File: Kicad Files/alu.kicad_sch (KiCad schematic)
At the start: 27 parts, among them U47 74LS245, U48 74LS283, U49 74LS283, U50 74LS86, U51 74LS86

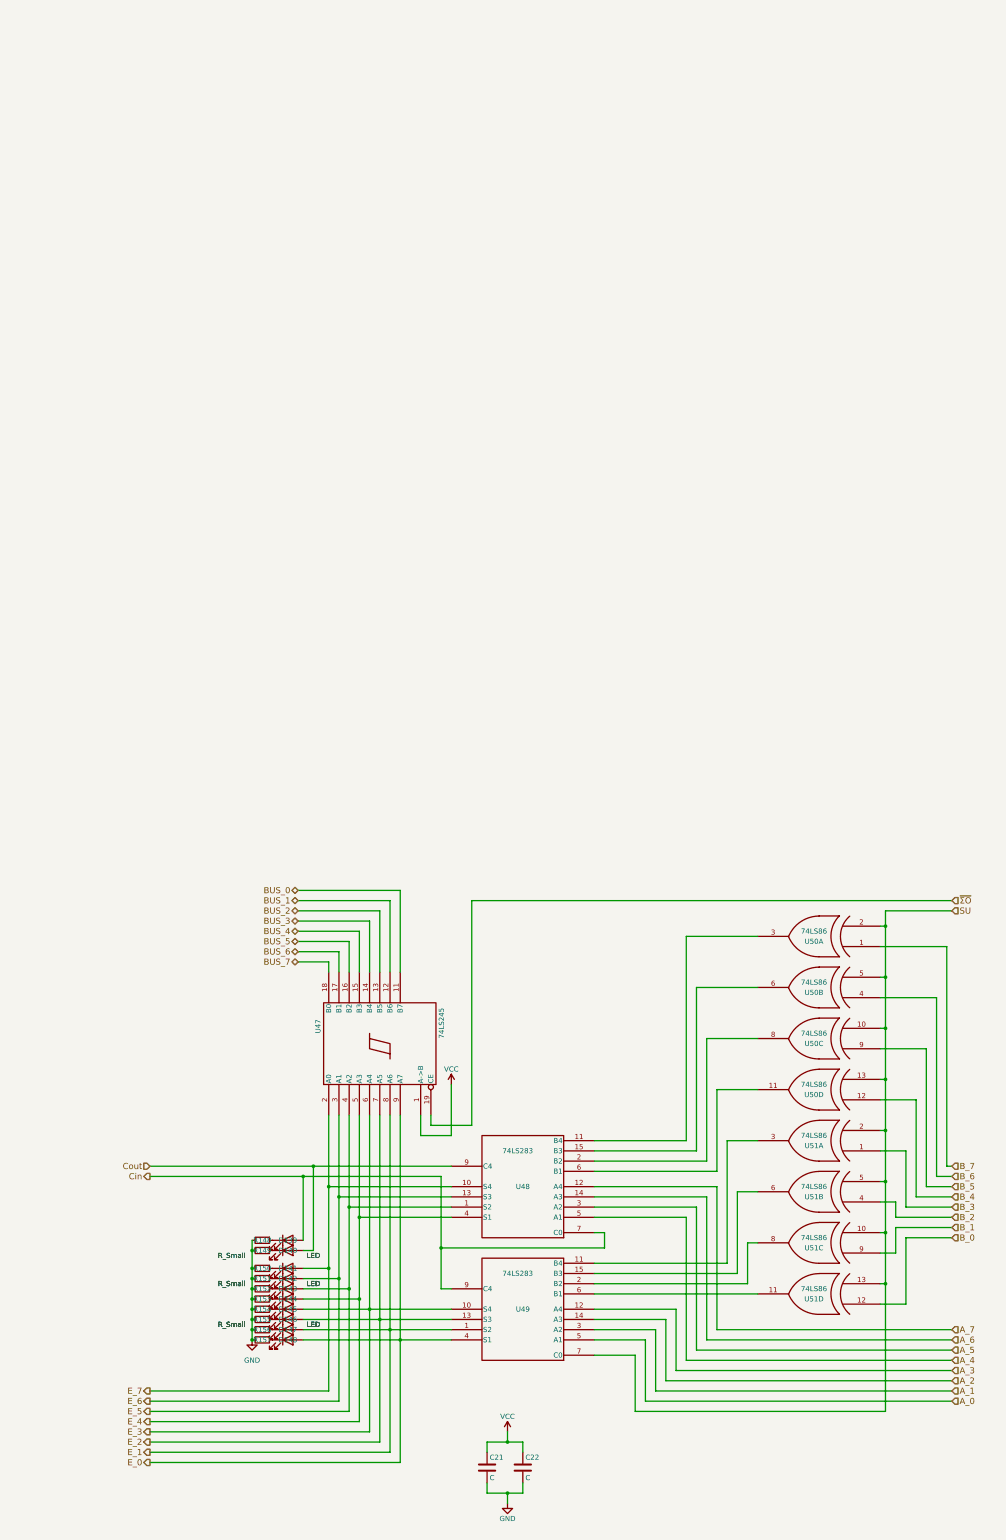
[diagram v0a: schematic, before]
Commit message: alu rework start
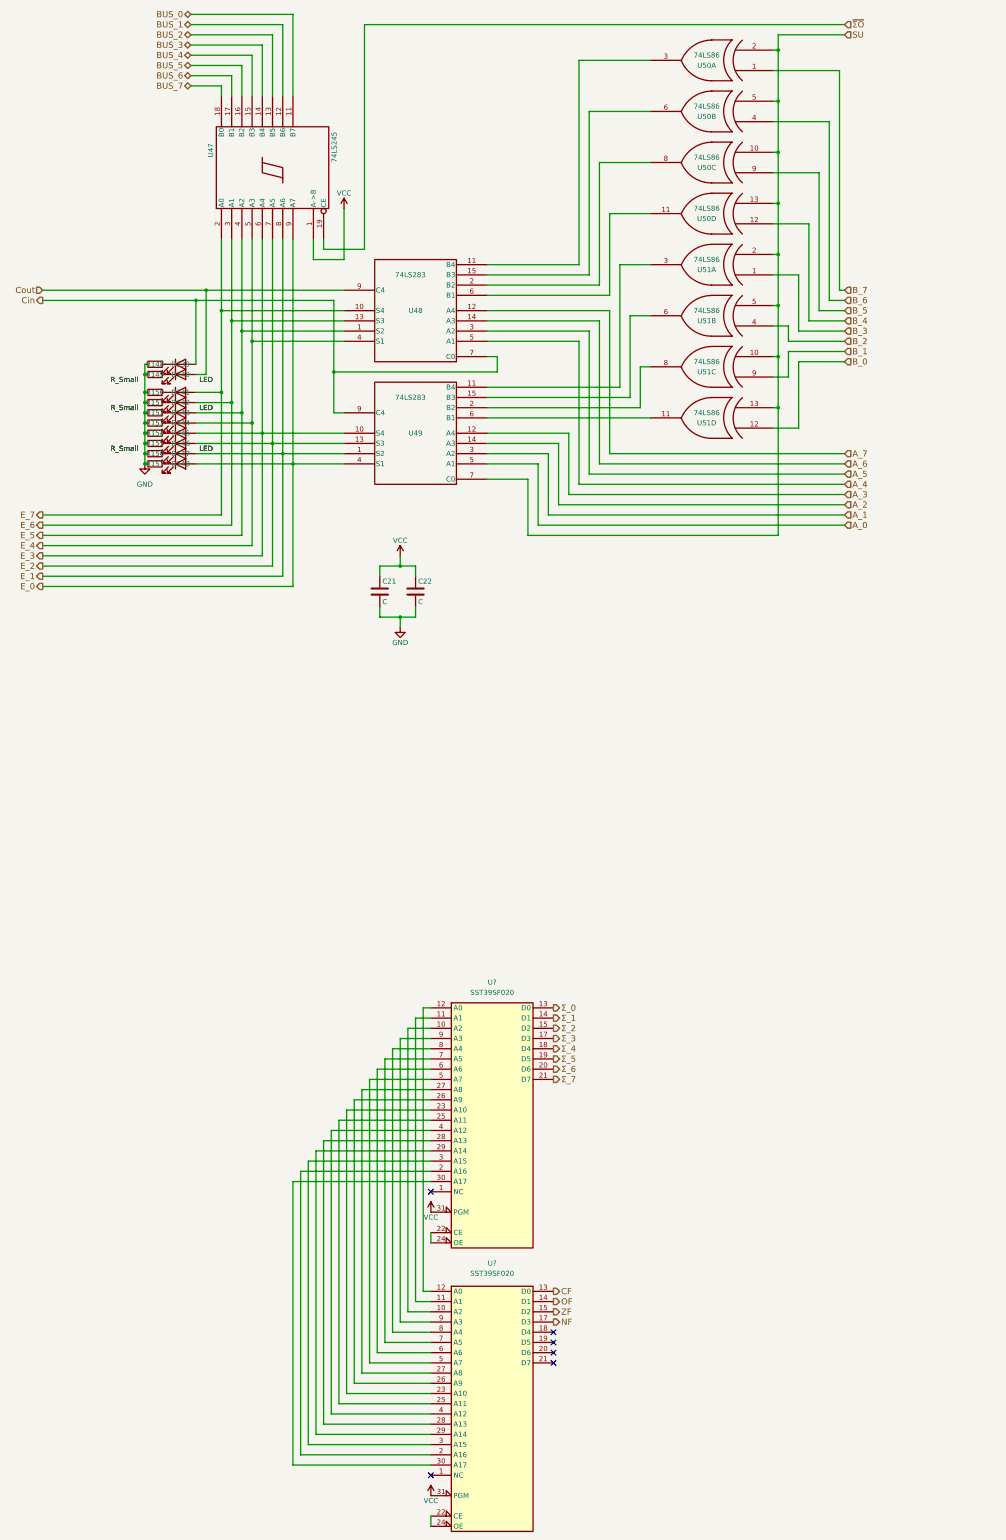
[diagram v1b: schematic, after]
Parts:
- added U? (x2): SST39SF020, symbol Memory_Flash:SST39SF020
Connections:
- net GND: now also U?.16 (GND), U?.16 (GND)
- net VCC: now also U?.31 (PGM), U?.31 (PGM), U?.32 (VCC), U?.32 (VCC)
- new net: U?.10 (A2), U?.10 (A2)
- new net: U?.11 (A1), U?.11 (A1)
- new net: U?.12 (A0), U?.12 (A0)
- new net: U?.2 (A16), U?.2 (A16)
- new net: U?.22 (CE), U?.24 (OE) (x2)
- new net: U?.23 (A10), U?.23 (A10)
- new net: U?.25 (A11), U?.25 (A11)
- new net: U?.26 (A9), U?.26 (A9)
- new net: U?.27 (A8), U?.27 (A8)
- new net: U?.28 (A13), U?.28 (A13)
- new net: U?.29 (A14), U?.29 (A14)
- new net: U?.3 (A15), U?.3 (A15)
- new net: U?.30 (A17), U?.30 (A17)
- new net: U?.4 (A12), U?.4 (A12)
- new net: U?.5 (A7), U?.5 (A7)
- new net: U?.6 (A6), U?.6 (A6)
- new net: U?.7 (A5), U?.7 (A5)
- new net: U?.8 (A4), U?.8 (A4)
- new net: U?.9 (A3), U?.9 (A3)
- new net CF: U?.13 (D0)
- new net NF: U?.17 (D3)
- new net OF: U?.14 (D1)
- new net ZF: U?.15 (D2)
- new net Σ_0: U?.13 (D0)
- new net Σ_1: U?.14 (D1)
- new net Σ_2: U?.15 (D2)
- new net Σ_3: U?.17 (D3)
- new net Σ_4: U?.18 (D4)
- new net Σ_5: U?.19 (D5)
- new net Σ_6: U?.20 (D6)
- new net Σ_7: U?.21 (D7)
- no-connect marks 0 -> 6
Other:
- moved on the sheet: C21, C22, D139, D140, D141, D142, D143, D144, D145, D146, D147, D148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
